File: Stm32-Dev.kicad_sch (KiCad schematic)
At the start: 23 parts, among them J1 Conn_ST_STDC14, J2 STDC14, U1 STM32F405RGTx, X1 25MHz

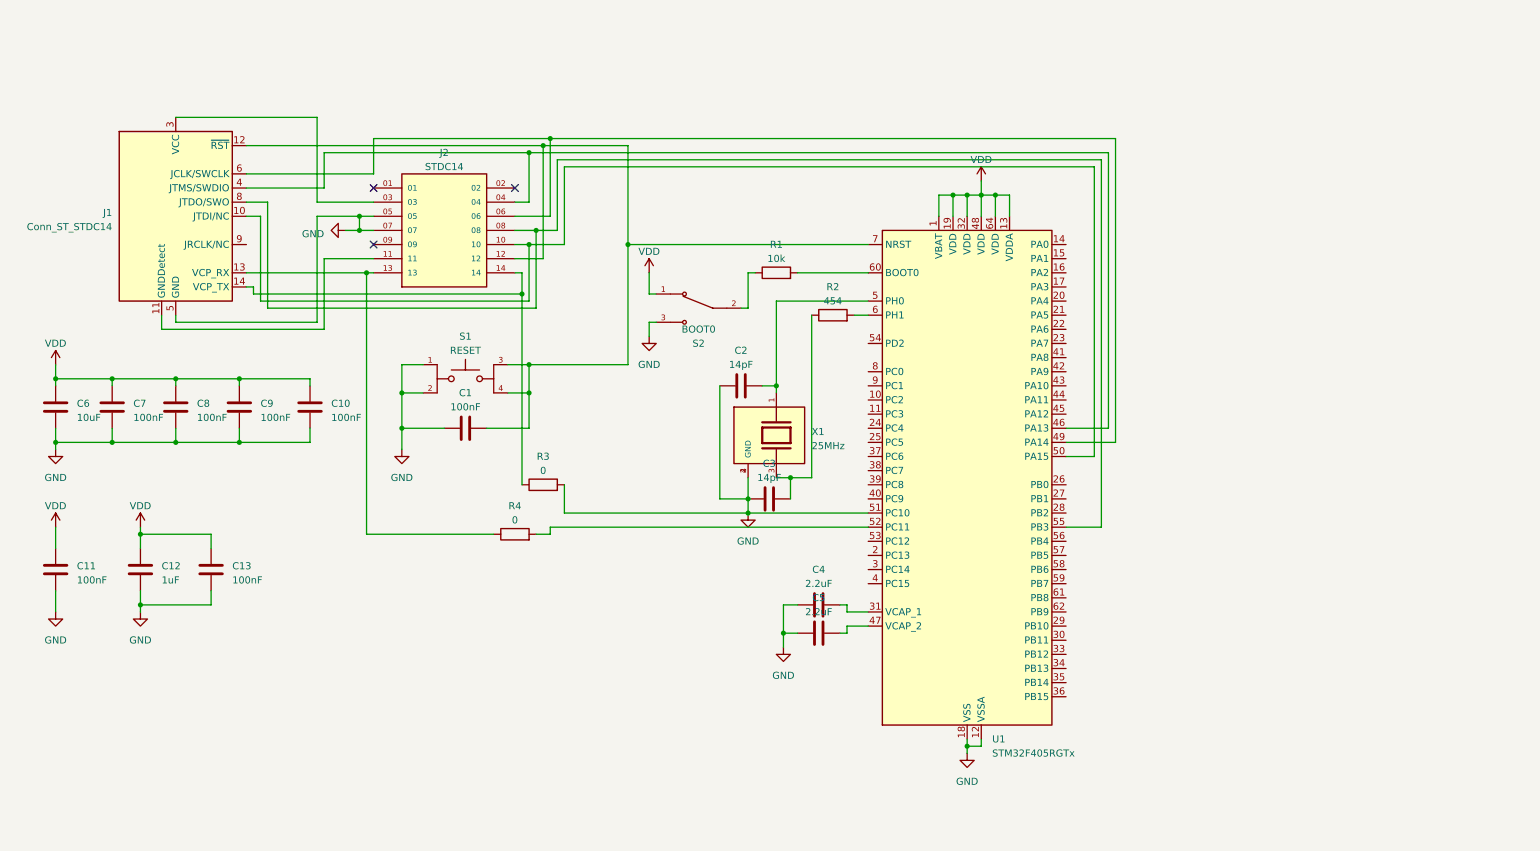
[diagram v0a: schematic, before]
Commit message: PCB start
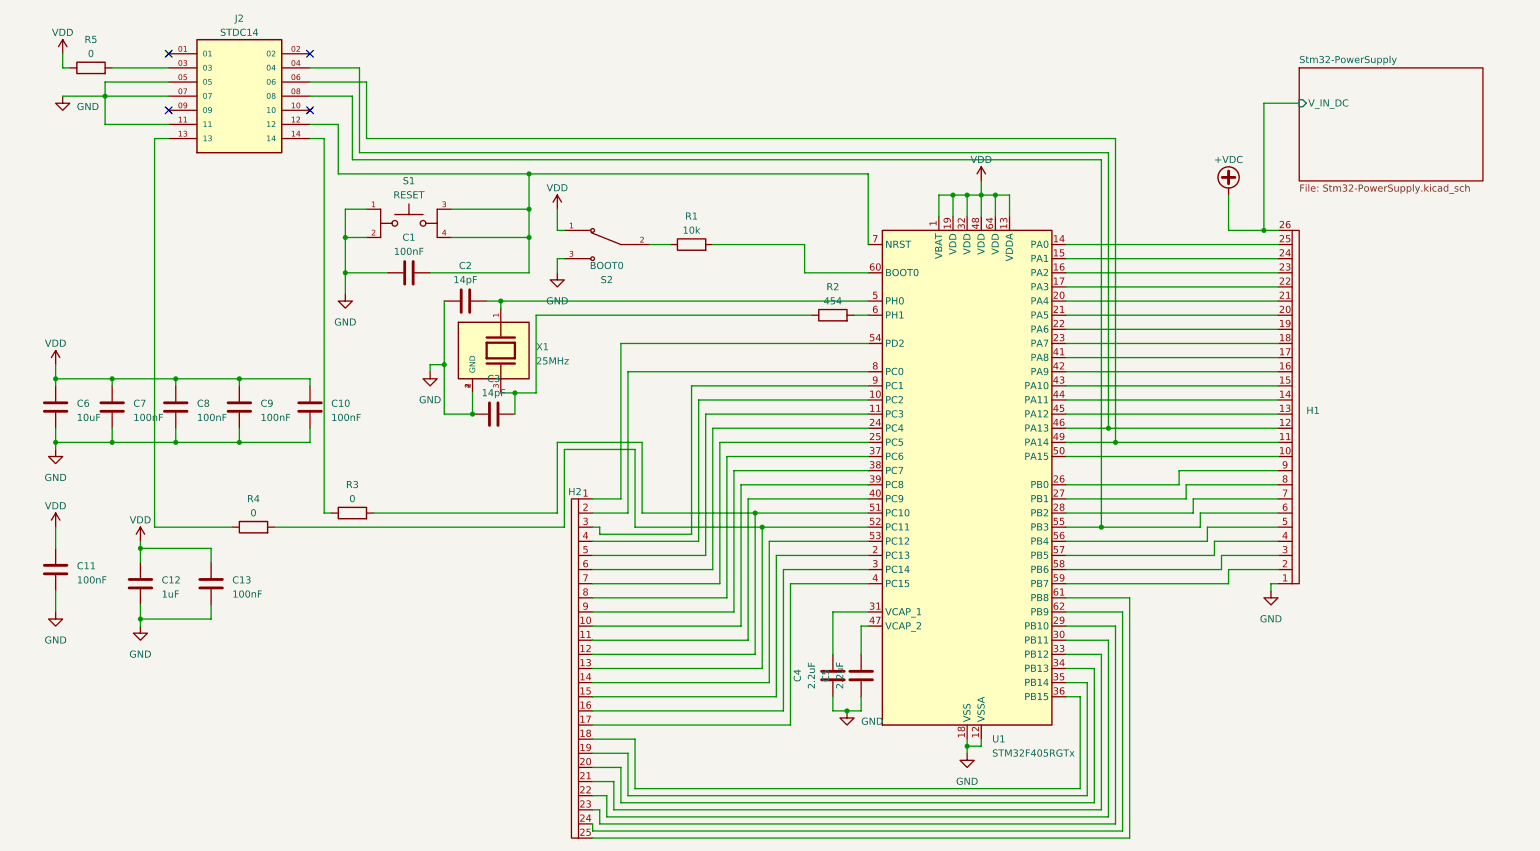
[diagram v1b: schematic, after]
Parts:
- removed J1: Conn_ST_STDC14, symbol Connector:Conn_ST_STDC14
- added H1: ~, 24_PIN_HEADER:HDRV26, symbol 24_PIN_HEADER:26_Header
- added H2: ~, 24_PIN_HEADER:HDRV25, symbol 24_PIN_HEADER:25_Header
- added R5: 0, Resistor_SMD:R_0805_2012Metric, symbol Device:R
- J2: footprint SAMTEC_FTSH-107-01-L-DV-K -> FTSH-107-01-L-DV-K:SAMTEC_FTSH-107-01-L-DV-K
- R2, R3, R4: footprint (none) -> Resistor_SMD:R_0805_2012Metric
- S1: footprint SW_TL3301AF160QG -> TL3301AF160QG:SW_TL3301AF160QG
- S2: footprint Button_Switch_THT:SW_E-Switch_EG1224_SPDT_Angled -> EG1215AA:SW_EG1215AA
- X1: footprint XTAL_ABM10W-25.0000MHZ-7-D1X-T3 -> ABM10W-25.0000MHZ-7-D1X-T3:XTAL_ABM10W-25.0000MHZ-7-D1X-T3
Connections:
- net GND: now also J2.11, H1.1; no longer R3.2, U1.51 (PC10)
- net VDD: now also R5.1
- net at U1.10 (PC2): now also H2.4
- net at U1.11 (PC3): now also H2.5
- net at U1.14 (PA0): now also H1.25
- net at U1.15 (PA1): now also H1.24
- net at U1.16 (PA2): now also H1.23
- net at U1.17 (PA3): now also H1.22
- net at U1.2 (PC13): now also H2.15
- net at U1.20 (PA4): now also H1.21
- net at U1.21 (PA5): now also H1.20
- net at U1.22 (PA6): now also H1.19
- net at U1.23 (PA7): now also H1.18
- net at U1.24 (PC4): now also H2.6
- net at U1.25 (PC5): now also H2.7
- net at U1.26 (PB0): now also H1.9
- net at U1.27 (PB1): now also H1.8
- net at U1.28 (PB2): now also H1.7
- net at U1.29 (PB10): now also H2.23
- net at U1.3 (PC14): now also H2.16
- net at U1.30 (PB11): now also H2.22
- net at U1.33 (PB12): now also H2.21
- net at U1.34 (PB13): now also H2.20
- net at U1.35 (PB14): now also H2.19
- net at U1.36 (PB15): now also H2.18
- net at U1.37 (PC6): now also H2.8
- net at U1.38 (PC7): now also H2.9
- net at U1.39 (PC8): now also H2.10
- net at U1.4 (PC15): now also H2.17
- net at U1.40 (PC9): now also H2.11
- net at U1.41 (PA8): now also H1.17
- net at U1.42 (PA9): now also H1.16
- net at U1.43 (PA10): now also H1.15
- net at U1.44 (PA11): now also H1.14
- net at U1.45 (PA12): now also H1.13
- net at J2.04, U1.46 (PA13): now also H1.12
- net at J2.06, U1.49 (PA14): now also H1.11
- net at U1.50 (PA15): now also H1.10; no longer J2.10
- net at R4.2, U1.52 (PC11): now also H2.13
- net at U1.53 (PC12): now also H2.14
- net at U1.54 (PD2): now also H2.1
- net at J2.08, U1.55 (PB3): now also H1.6
- net at U1.56 (PB4): now also H1.5
- net at U1.57 (PB5): now also H1.4
- net at U1.58 (PB6): now also H1.3
- net at U1.59 (PB7): now also H1.2
- net at U1.61 (PB8): now also H2.25
- net at U1.62 (PB9): now also H2.24
- net at U1.8 (PC0): now also H2.2
- net at U1.9 (PC1): now also H2.3
- net at J2.03: now also R5.2
- new net: H2.12, R3.2, U1.51 (PC10)
- new net +VDC: H1.26
- no-connect marks 3 -> 4
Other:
- added sheet Stm32-PowerSupply (Stm32-PowerSupply.kicad_sch)
- moved on the sheet: C1, C12, C13, C2, C3, C4, C5, J2, R1, R3, R4, S1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
